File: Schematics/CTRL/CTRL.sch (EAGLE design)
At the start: 48 parts

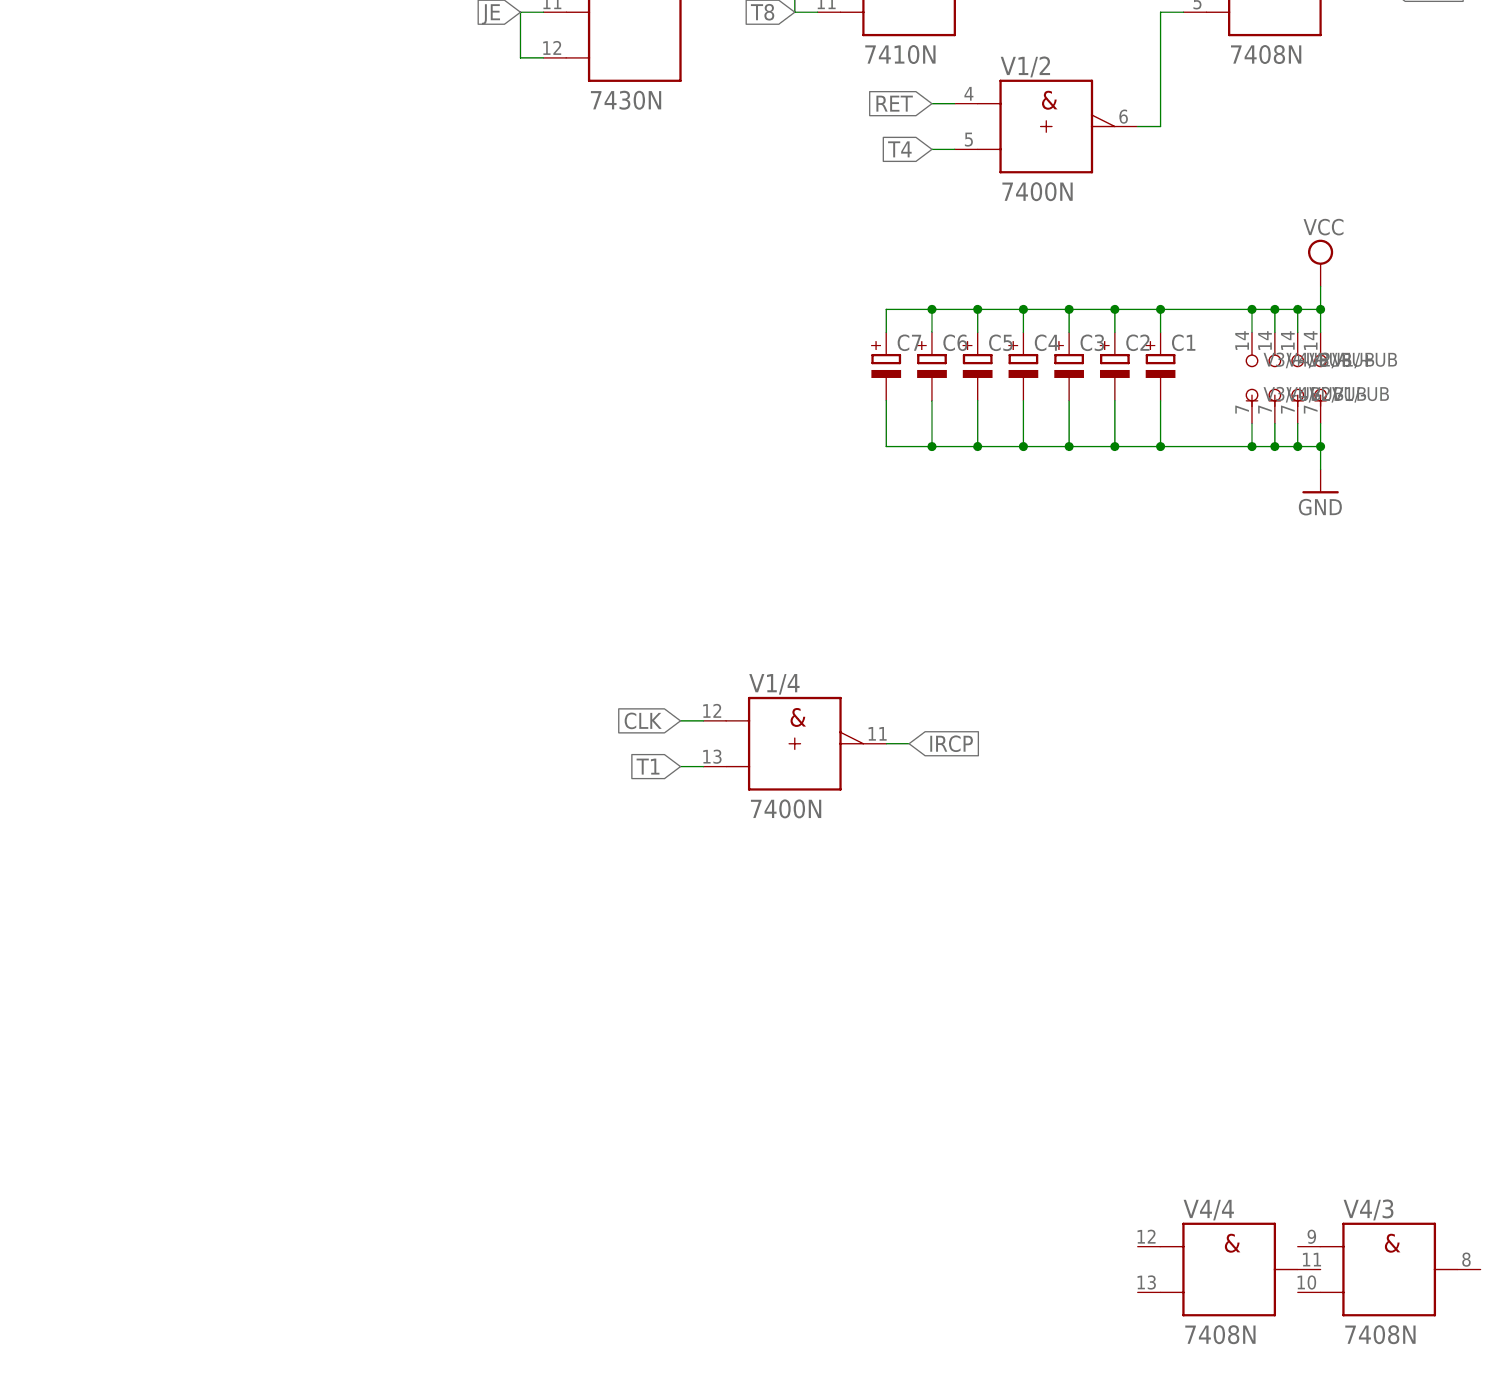
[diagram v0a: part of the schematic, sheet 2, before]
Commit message: LDO
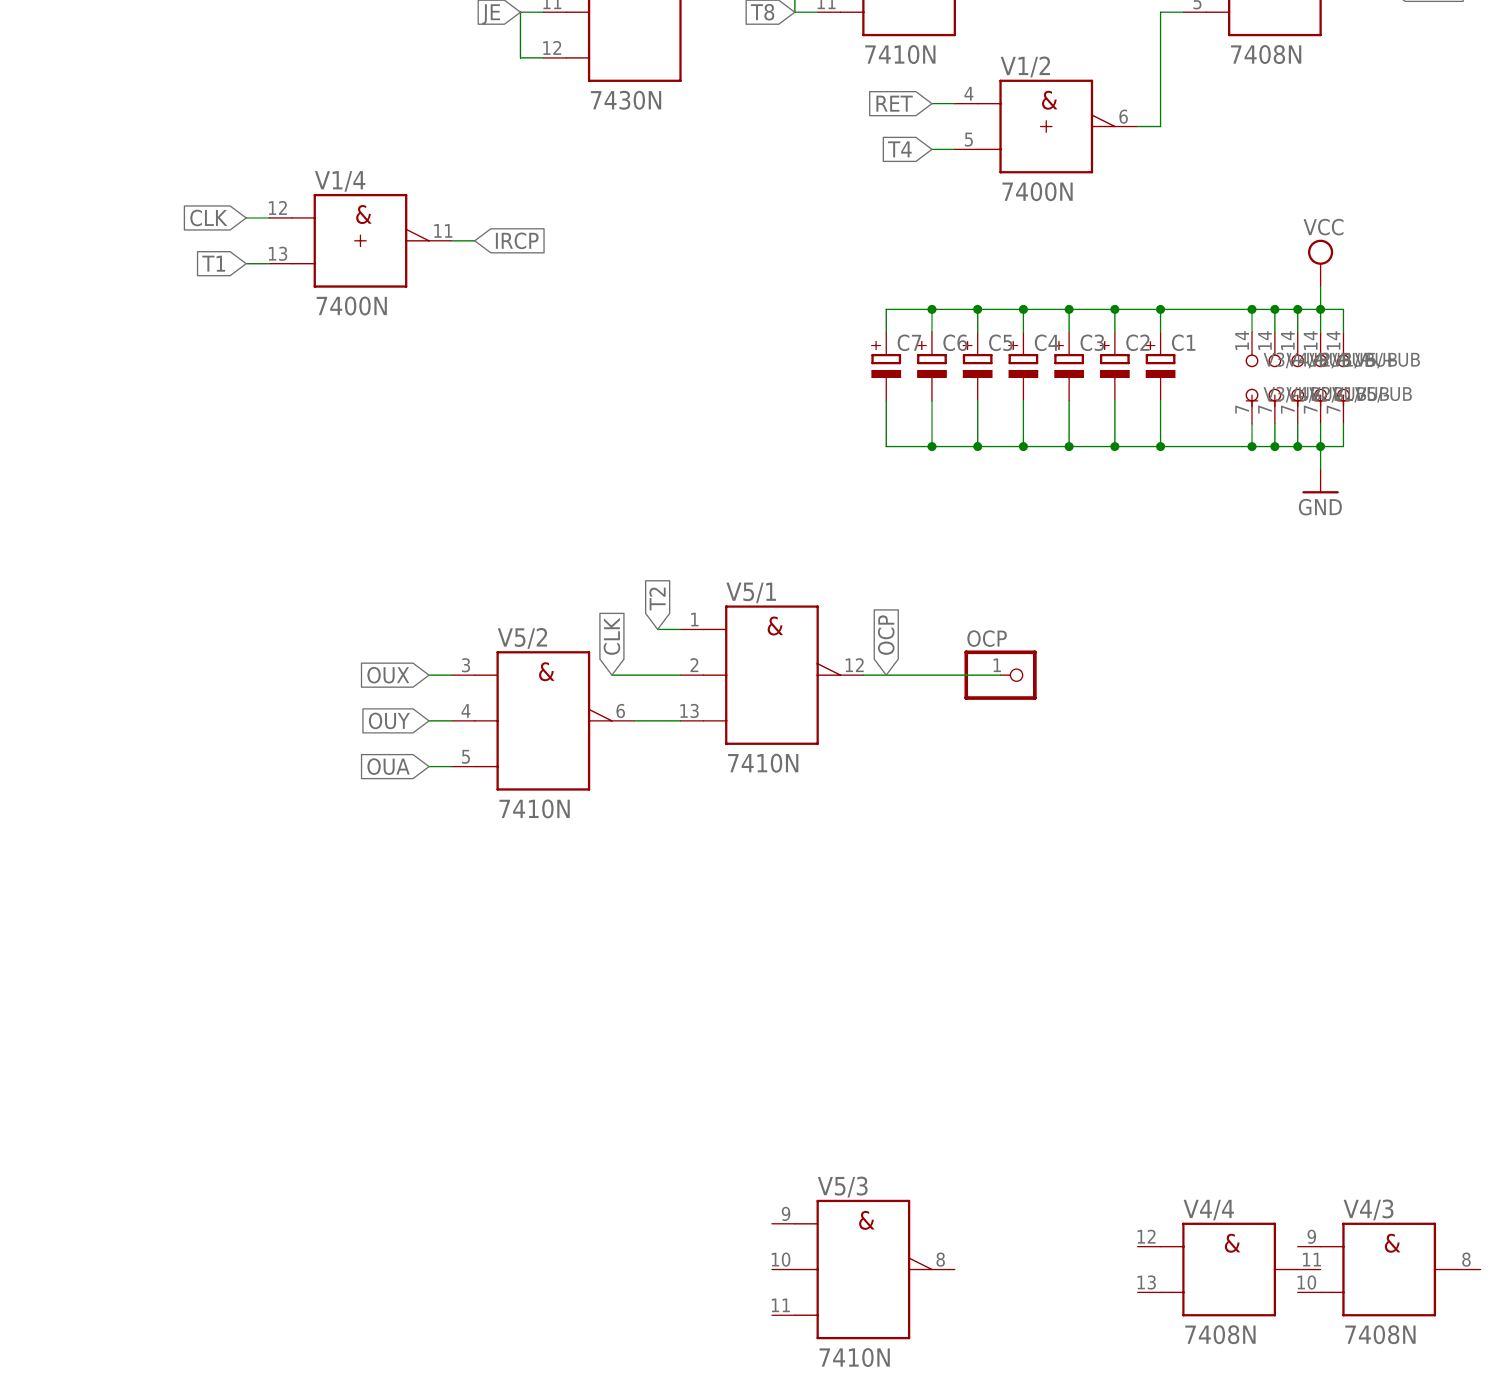
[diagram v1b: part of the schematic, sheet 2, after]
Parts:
- added OCP: (no value), pinhead:PINHD-1X1
- added V5: 7410N, 74ttl-din:7410N
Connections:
- new net N$6: V5/1.C, V5/2.Y
- new net OCP: OCP.1, V5/1.Y
- net CLK: now also V5/1.B
- net GND: now also V5/-UB.-UB
- net OUA: now also V5/2.C
- net OUX: now also V5/2.A
- net OUY: now also V5/2.B
- net T2: now also V5/1.A
- net VCC: now also V5/+UB.+UB
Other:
- moved on the sheet: V1/4
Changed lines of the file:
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@@
 <drawing>
 <settings>
-<setting alwaysvectorfont="yes"/>
+<setting alwaysvectorfont="no"/>
 <setting verticaltext="up"/>
 </settings>
@@
 <part name="ALU-OP1" library="pinhead" library_urn="urn:adsk.eagle:library:325" deviceset="PINHD-1X5" device="" package3d_urn="urn:adsk.eagle:package:22469/2"/>
 <part name="ALU-OP0" library="pinhead" library_urn="urn:adsk.eagle:library:325" deviceset="PINHD-1X30" device="" package3d_urn="urn:adsk.eagle:package:22460/2"/>
+<part name="V5" library="74ttl-din" library_urn="urn:adsk.eagle:library:84" deviceset="74*10" device="N" package3d_urn="urn:adsk.eagle:package:16407/2"/>
+<part name="OCP" library="pinhead" library_urn="urn:adsk.eagle:library:325" deviceset="PINHD-1X1" device="" package3d_urn="urn:adsk.eagle:package:22485/2"/>
 </parts>
 <sheets>
@@
 <attribute name="VALUE" x="327.66" y="217.805" size="2.032" layer="96"/>
 </instance>
-<instance part="V1" gate="/4" x="304.8" y="109.22" smashed="yes">
-<attribute name="NAME" x="299.72" y="114.935" size="2.032" layer="95"/>
-<attribute name="VALUE" x="299.72" y="100.965" size="2.032" layer="96"/>
+<instance part="V1" gate="/4" x="256.54" y="165.1" smashed="yes">
+<attribute name="NAME" x="251.46" y="170.815" size="2.032" layer="95"/>
+<attribute name="VALUE" x="251.46" y="156.845" size="2.032" layer="96"/>
 </instance>
 <instance part="V2" gate="/1" x="322.58" y="243.84" smashed="yes">
@@
 <attribute name="NAME" x="161.29" y="108.585" size="1.778" layer="95" rot="R180"/>
 <attribute name="VALUE" x="161.29" y="190.5" size="1.778" layer="96" rot="R180"/>
+</instance>
+<instance part="V5" gate="/1" x="302.26" y="116.84" smashed="yes">
+<attribute name="NAME" x="297.18" y="125.095" size="2.032" layer="95"/>
+<attribute name="VALUE" x="297.18" y="106.045" size="2.032" layer="96"/>
+</instance>
+<instance part="V5" gate="/2" x="276.86" y="111.76" smashed="yes">
+<attribute name="NAME" x="271.78" y="120.015" size="2.032" layer="95"/>
+<attribute name="VALUE" x="271.78" y="100.965" size="2.032" layer="96"/>
+</instance>
+<instance part="V5" gate="/3" x="312.42" y="50.8" smashed="yes">
+<attribute name="NAME" x="307.34" y="59.055" size="2.032" layer="95"/>
+<attribute name="VALUE" x="307.34" y="40.005" size="2.032" layer="96"/>
+</instance>
+<instance part="OCP" gate="G$1" x="330.2" y="116.84" smashed="yes">
+<attribute name="NAME" x="323.85" y="120.015" size="1.778" layer="95"/>
+<attribute name="VALUE" x="323.85" y="111.76" size="1.778" layer="96"/>
+</instance>
+<instance part="V5" gate="/+UB" x="365.76" y="152.4" smashed="yes">
+<attribute name="NAME" x="367.03" y="151.13" size="1.524" layer="95"/>
+</instance>
+<instance part="V5" gate="/-UB" x="365.76" y="147.32" smashed="yes">
+<attribute name="NAME" x="367.03" y="147.32" size="1.524" layer="95"/>
 </instance>
 </instances>
@@
 <pinref part="ALU-T" gate="A" pin="5"/>
 <label x="162.56" y="210.82" size="1.778" layer="95" xref="yes"/>
+</segment>
+<segment>
+<pinref part="V5" gate="/1" pin="A"/>
+<wire x1="289.56" y1="121.92" x2="292.1" y2="121.92" width="0.1524" layer="91"/>
+<label x="289.56" y="121.92" size="1.778" layer="95" rot="R90" xref="yes"/>
 </segment>
 </net>
@@
 <wire x1="320.04" y1="154.94" x2="320.04" y2="157.48" width="0.1524" layer="91"/>
 <junction x="320.04" y="157.48"/>
+<pinref part="V5" gate="/+UB" pin="+UB"/>
+<wire x1="365.76" y1="154.94" x2="365.76" y2="157.48" width="0.1524" layer="91"/>
+<wire x1="365.76" y1="157.48" x2="363.22" y2="157.48" width="0.1524" layer="91"/>
 </segment>
 <segment>
@@
 <wire x1="320.04" y1="147.32" x2="320.04" y2="142.24" width="0.1524" layer="91"/>
 <junction x="320.04" y="142.24"/>
+<pinref part="V5" gate="/-UB" pin="-UB"/>
+<wire x1="365.76" y1="144.78" x2="365.76" y2="142.24" width="0.1524" layer="91"/>
+<wire x1="365.76" y1="142.24" x2="363.22" y2="142.24" width="0.1524" layer="91"/>
 </segment>
 <segment>
@@
 <segment>
 <pinref part="V1" gate="/4" pin="A"/>
-<wire x1="292.1" y1="111.76" x2="294.64" y2="111.76" width="0.1524" layer="91"/>
-<label x="292.1" y="111.76" size="1.778" layer="95" rot="R180" xref="yes"/>
+<wire x1="243.84" y1="167.64" x2="246.38" y2="167.64" width="0.1524" layer="91"/>
+<label x="243.84" y="167.64" size="1.778" layer="95" rot="R180" xref="yes"/>
+</segment>
+<segment>
+<pinref part="V5" gate="/1" pin="B"/>
+<wire x1="284.48" y1="116.84" x2="292.1" y2="116.84" width="0.1524" layer="91"/>
+<label x="284.48" y="116.84" size="1.778" layer="95" rot="R90" xref="yes"/>
 </segment>
 </net>
@@
 <label x="17.78" y="185.42" size="1.778" layer="95" xref="yes"/>
 </segment>
+<segment>
+<pinref part="V5" gate="/2" pin="A"/>
+<wire x1="264.16" y1="116.84" x2="266.7" y2="116.84" width="0.1524" layer="91"/>
+<label x="264.16" y="116.84" size="1.778" layer="95" rot="R180" xref="yes"/>
+</segment>
 </net>
 <net name="OUY" class="0">
@@
 <label x="33.02" y="182.88" size="1.778" layer="95" xref="yes"/>
 </segment>
+<segment>
+<pinref part="V5" gate="/2" pin="B"/>
+<wire x1="264.16" y1="111.76" x2="266.7" y2="111.76" width="0.1524" layer="91"/>
+<label x="264.16" y="111.76" size="1.778" layer="95" rot="R180" xref="yes"/>
+</segment>
 </net>
 <net name="CMY" class="0">
@@
 <segment>
 <pinref part="V1" gate="/4" pin="B"/>
-<wire x1="292.1" y1="106.68" x2="294.64" y2="106.68" width="0.1524" layer="91"/>
-<label x="292.1" y="106.68" size="1.778" layer="95" rot="R180" xref="yes"/>
+<wire x1="243.84" y1="162.56" x2="246.38" y2="162.56" width="0.1524" layer="91"/>
+<label x="243.84" y="162.56" size="1.778" layer="95" rot="R180" xref="yes"/>
 </segment>
 </net>
@@
 <label x="175.26" y="182.88" size="1.778" layer="95" xref="yes"/>
 </segment>
+<segment>
+<pinref part="V5" gate="/2" pin="C"/>
+<wire x1="264.16" y1="106.68" x2="266.7" y2="106.68" width="0.1524" layer="91"/>
+<label x="264.16" y="106.68" size="1.778" layer="95" rot="R180" xref="yes"/>
+</segment>
 </net>
 <net name="CMA" class="0">
@@
 <segment>
 <pinref part="V1" gate="/4" pin="Y"/>
-<wire x1="317.5" y1="109.22" x2="314.96" y2="109.22" width="0.1524" layer="91"/>
-<label x="317.5" y="109.22" size="1.778" layer="95" xref="yes"/>
-</segment>
-</net>
+<wire x1="269.24" y1="165.1" x2="266.7" y2="165.1" width="0.1524" layer="91"/>
+<label x="269.24" y="165.1" size="1.778" layer="95" xref="yes"/>
+</segment>
+</net>
+<net name="OCP" class="0">
+<segment>
+<pinref part="V5" gate="/1" pin="Y"/>
+<label x="314.96" y="116.84" size="1.778" layer="95" rot="R90" xref="yes"/>
+<pinref part="OCP" gate="G$1" pin="1"/>
+<wire x1="327.66" y1="116.84" x2="312.42" y2="116.84" width="0.1524" layer="91"/>
+</segment>
+</net>
+<net name="N$6" class="0">
+<segment>
+<pinref part="V5" gate="/2" pin="Y"/>
+<pinref part="V5" gate="/1" pin="C"/>
+<wire x1="287.02" y1="111.76" x2="292.1" y2="111.76" width="0.1524" layer="91"/>
+</segment>
+</net>
